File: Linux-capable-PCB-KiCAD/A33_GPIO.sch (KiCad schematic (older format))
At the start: 44 parts, among them J1 UART_CONN, J2 GPIO_CONN, J3 USB_A, J4 USB_A, J5 Micro_SD_Card_Det, J6 MIC_DIFF_IN, Q1 Q_PMOS_GSD, Q2 BC547, U1 A33, U2 MMA8425Q_Gsensor, U3 SRV05-4, U4 MIPI_DSI_Raspberry, U5 SRV05-4, U6 SRV05-4, Y1 24MHz, Y2 32.768kHz

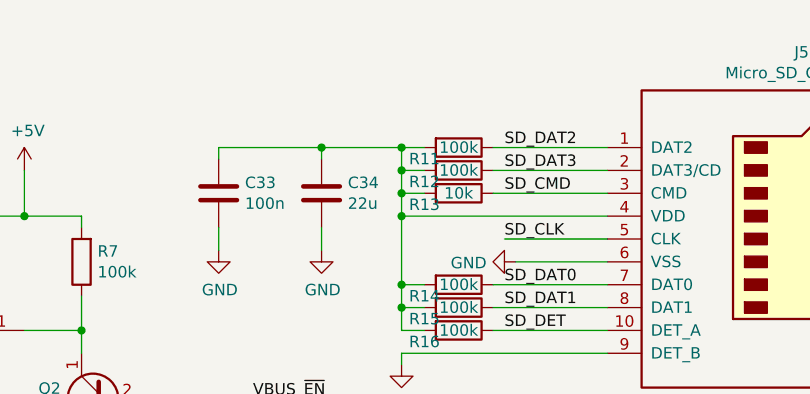
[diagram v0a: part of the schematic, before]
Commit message: Od kuce
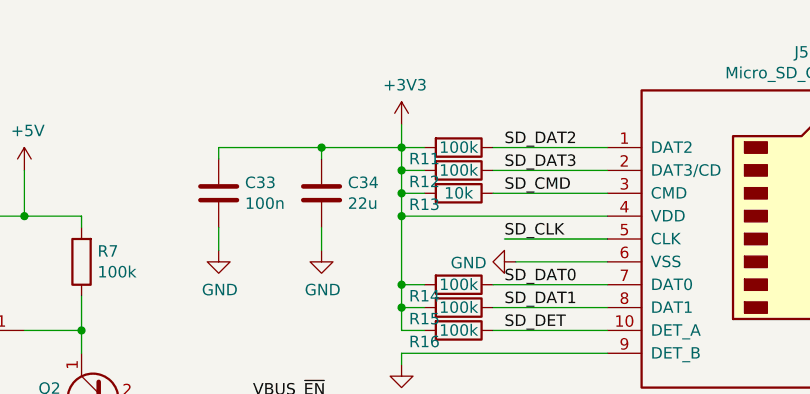
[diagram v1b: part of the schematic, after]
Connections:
- net +3V3: now also C33.1, C34.1, J5.4 (VDD), R11.2, R12.2, R13.2, R14.2, R15.2, R16.2
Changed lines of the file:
@@
 Wire Wire Line
 	6400 2200 6400 2550
-Wire Wire Line
-	8000 1100 8350 1100
 Connection ~ 8000 1100
 Connection ~ 8350 1100
@@
 Wire Wire Line
 	6850 7550 6850 7300
+$Comp
+L power:+3V3 #PWR?
+U 1 1 62CFA384
+P 8350 1000
+F 0 "#PWR?" H 8350 850 50  0001 C CNN
+F 1 "+3V3" H 8365 1173 50  0000 C CNN
+F 2 "" H 8350 1000 50  0001 C CNN
+F 3 "" H 8350 1000 50  0001 C CNN
+	1    8350 1000
+	1    0    0    -1
+$EndComp
+Wire Wire Line
+	8000 1100 8350 1100
+Wire Wire Line
+	8350 1000 8350 1100
 $EndSCHEMATC

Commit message: Revert "Od kuce"
This reverts commit 2bece482254f98a379437a0618b8cb6327aa6629.
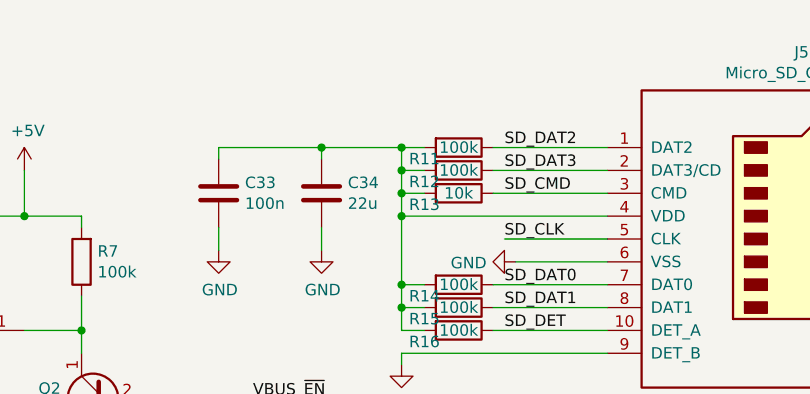
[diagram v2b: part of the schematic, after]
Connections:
- net +3V3: no longer C33.1, C34.1, J5.4 (VDD), R11.2, R12.2, R13.2, R14.2, R15.2, R16.2
- new net: C33.1, C34.1, J5.4 (VDD), R11.2, R12.2, R13.2, R14.2, R15.2, R16.2
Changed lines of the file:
@@
 Wire Wire Line
 	6400 2200 6400 2550
+Wire Wire Line
+	8000 1100 8350 1100
 Connection ~ 8000 1100
 Connection ~ 8350 1100
@@
 Wire Wire Line
 	6850 7550 6850 7300
-$Comp
-L power:+3V3 #PWR?
-U 1 1 62CFA384
-P 8350 1000
-F 0 "#PWR?" H 8350 850 50  0001 C CNN
-F 1 "+3V3" H 8365 1173 50  0000 C CNN
-F 2 "" H 8350 1000 50  0001 C CNN
-F 3 "" H 8350 1000 50  0001 C CNN
-	1    8350 1000
-	1    0    0    -1
-$EndComp
-Wire Wire Line
-	8000 1100 8350 1100
-Wire Wire Line
-	8350 1000 8350 1100
 $EndSCHEMATC
